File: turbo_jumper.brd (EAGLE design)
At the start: 72.4 x 50.5 mm, 20 parts, among them J1 10090926-P264XLF, K1 G6K-2P, X1 E74

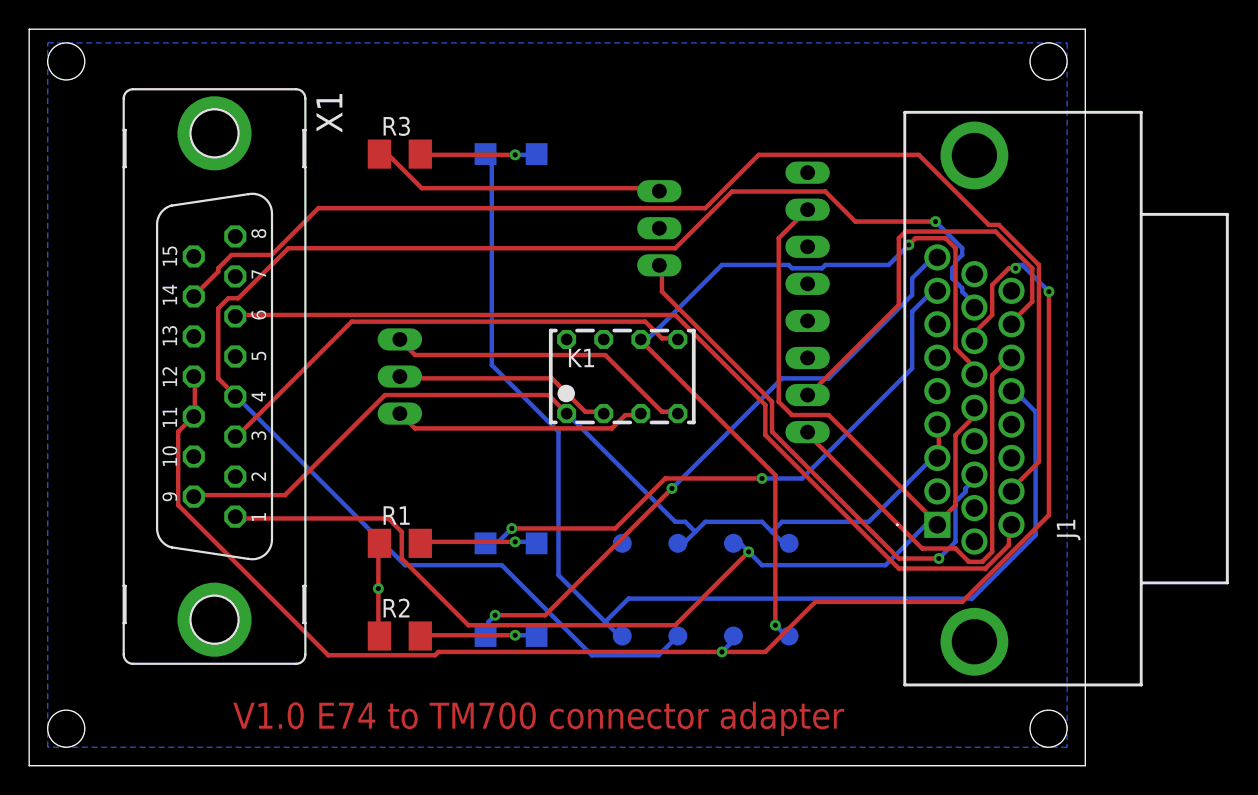
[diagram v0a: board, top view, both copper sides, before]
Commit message: up
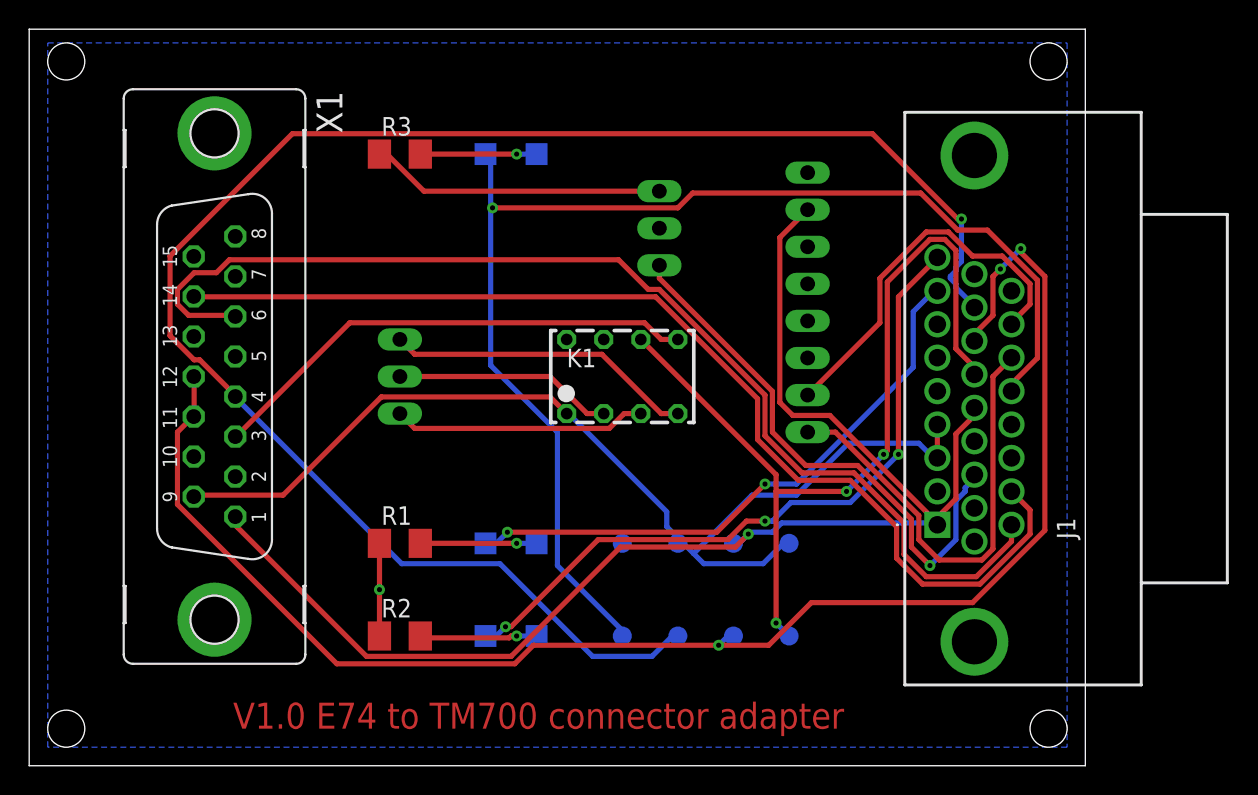
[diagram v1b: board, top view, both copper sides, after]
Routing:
- net ALARM+: track 63.6 -> 77.4 mm
- net NORM+: track 105.6 -> 117.3 mm
- net ALARM-: track 81.5 -> 73.2 mm
- net START-: track 65.8 -> 72.7 mm
- net REMOTE_ACTIVE: track 79.7 -> 85.7 mm, vias 0 -> 1
- net ERROR: track 43.1 -> 48.0 mm, vias 2 -> 3
- net NORM-: track 103.5 -> 105.9 mm
- net D-: track 28.2 -> 26.4 mm
- net AO1: track 36.4 -> 37.8 mm
- net NOT_NORM: track 58.7 -> 60.1 mm, vias 2 -> 3
- net D+: track 30.6 -> 31.2 mm
